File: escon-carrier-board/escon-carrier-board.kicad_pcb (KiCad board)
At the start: 2 copper layers, 35.6 x 26.7 mm, 6 parts, among them J1 Conn_01x06

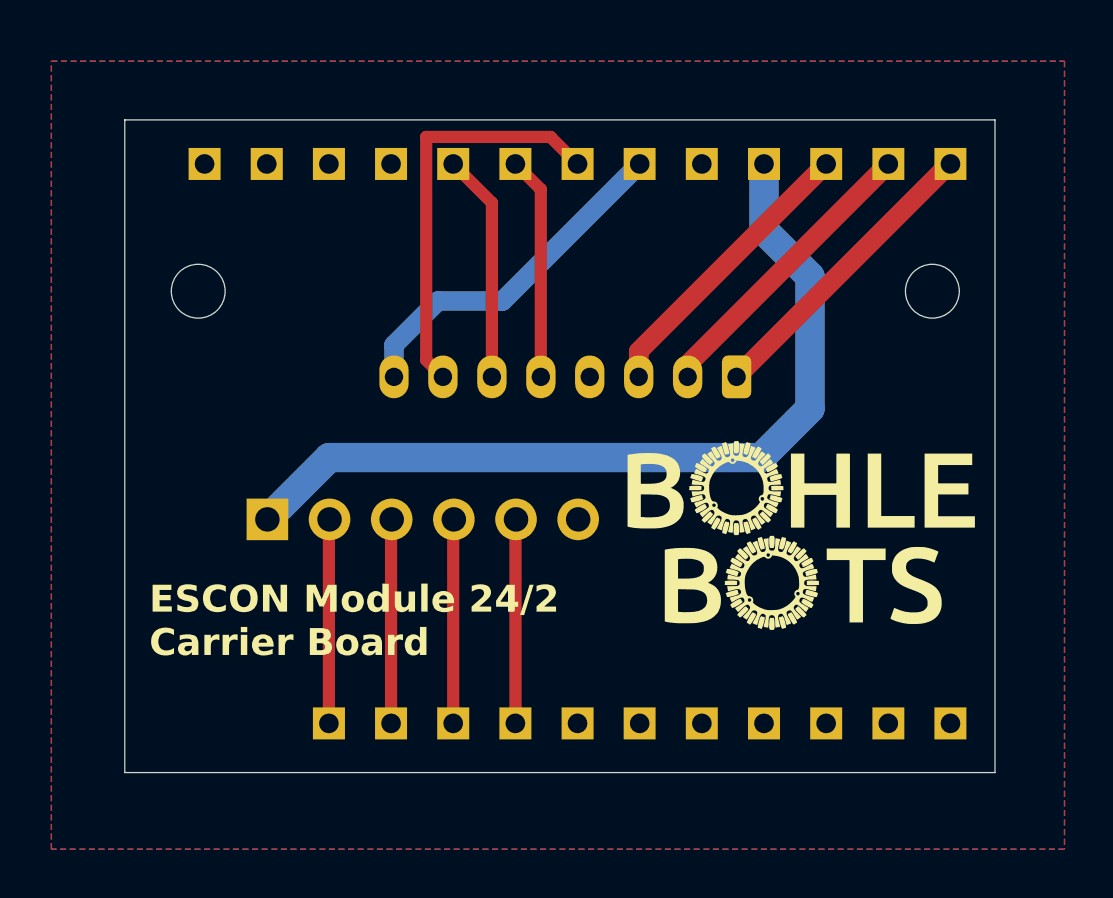
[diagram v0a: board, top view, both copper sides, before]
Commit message: V5.0
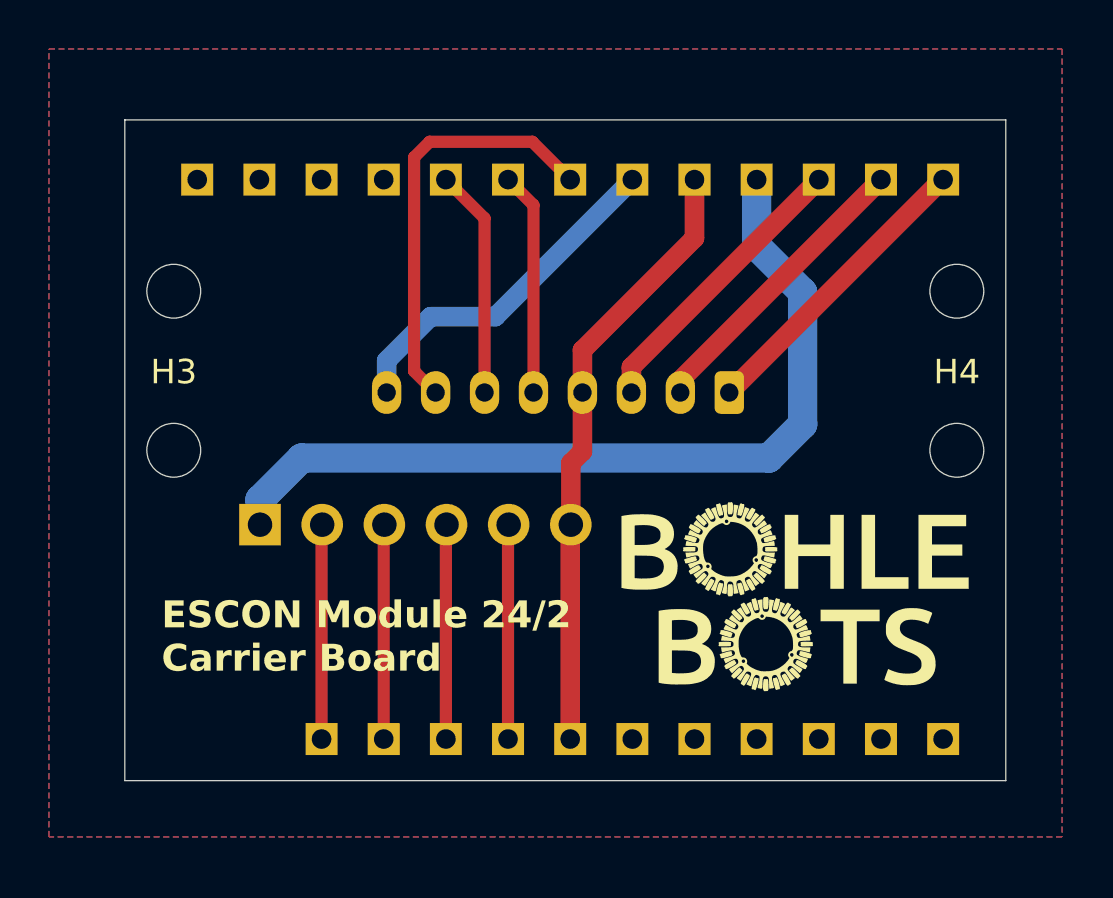
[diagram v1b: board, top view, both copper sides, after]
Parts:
- added G***: LOGO, BohleBots:logo_klein, B.Cu at (27.2, 19.5)
- added H3: MountingHole, MountingHole:MountingHole_2.2mm_M2, F.Cu at (2.00, 13.5)
- added H4: MountingHole, MountingHole:MountingHole_2.2mm_M2, F.Cu at (34.0, 13.5)
- moved G*** 2.51 mm to (27.2, 19.5)
- moved H1 1.00 mm to (34.0, 7.00)
- moved H2 1.00 mm to (2.00, 7.00)
- moved ESCON1 0.71 mm to (18.2, 15.1)
- moved JP1 0.71 mm to (24.7, 11.1)
- moved J1 0.37 mm to (5.53, 16.5)
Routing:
- net GND: track 0.00 -> 25.0 mm
- net Net-(ESCON1-H1): track 16.7 -> 17.3 mm
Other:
- board size 35.6 x 26.7 mm -> 36 x 27 mm
